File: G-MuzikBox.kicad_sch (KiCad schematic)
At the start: 2 parts, among them IC1 AK4458VN, U1 ORANGE_PI_CM4

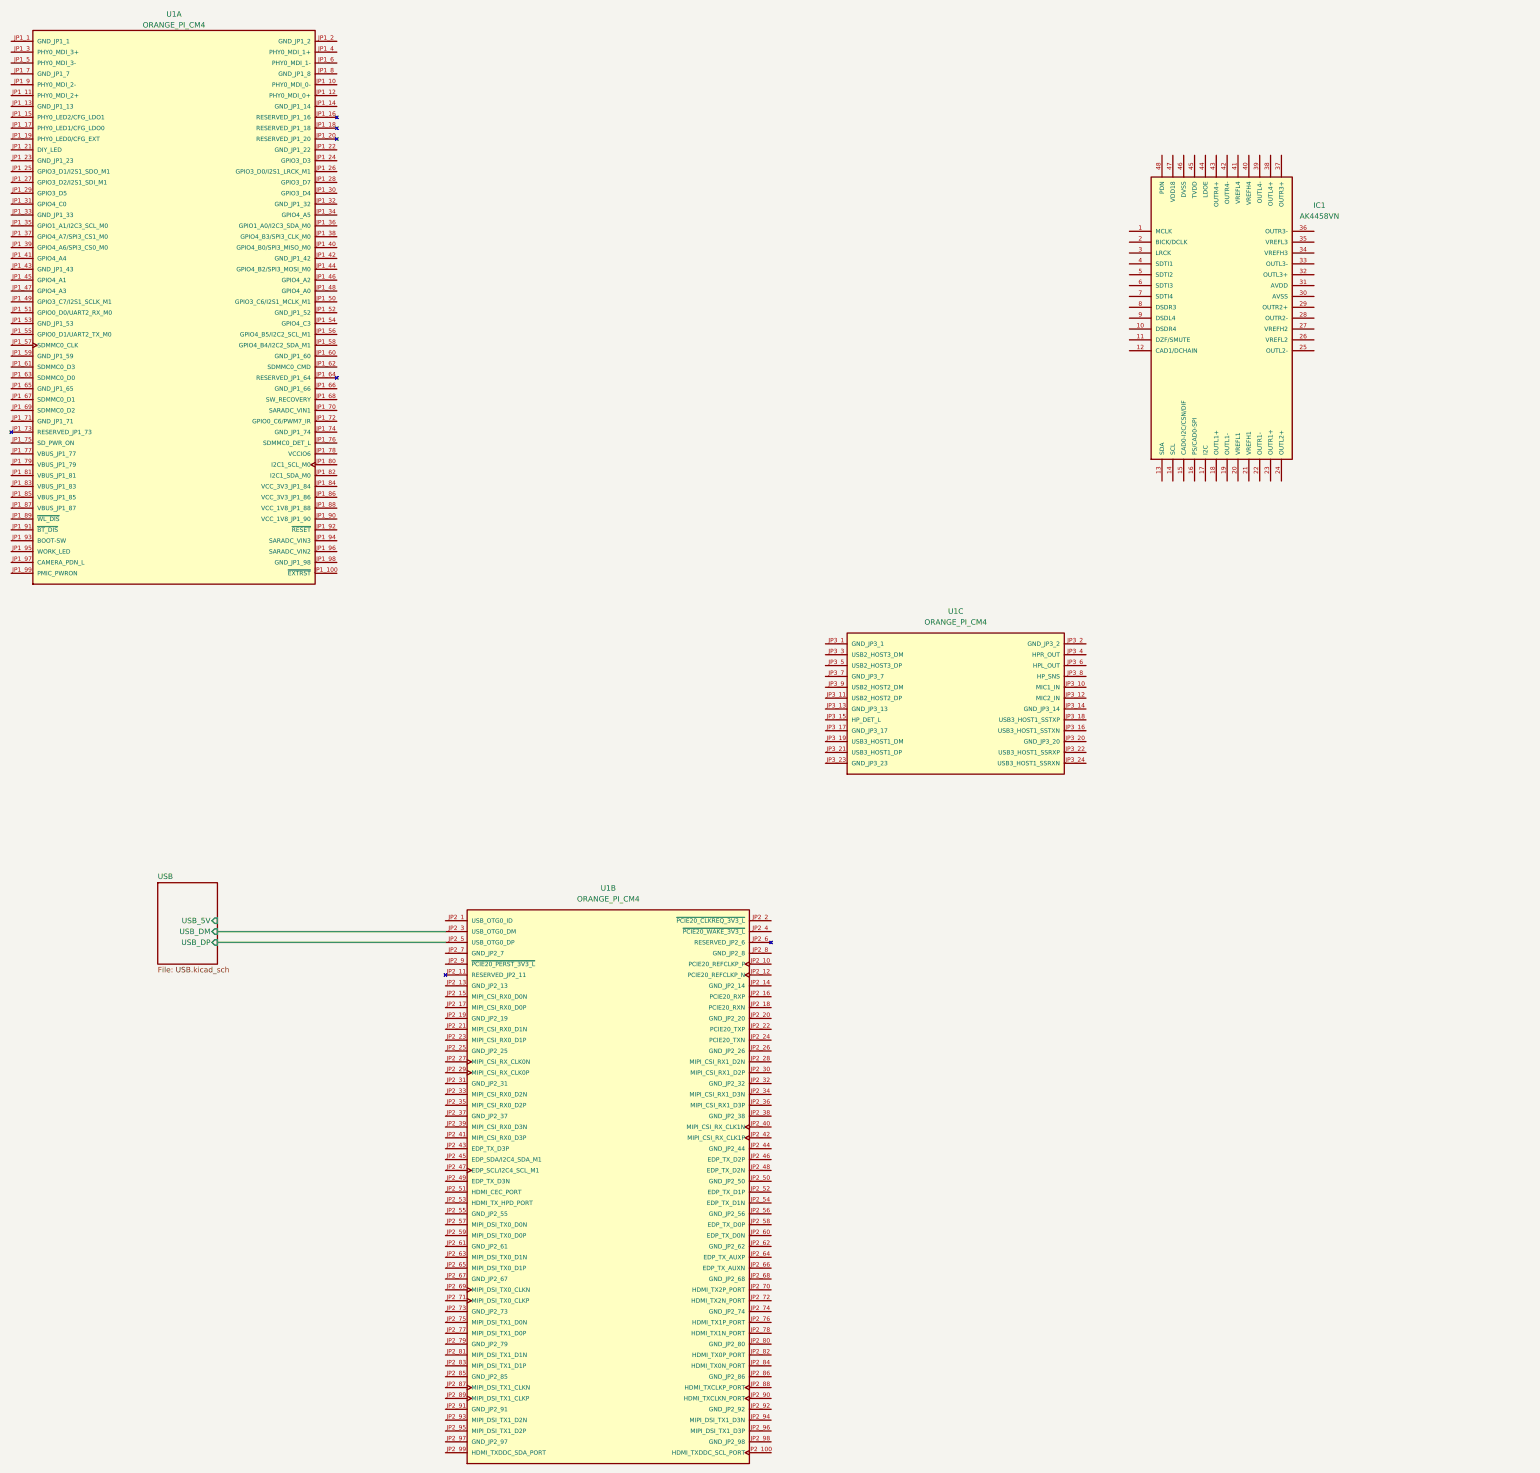
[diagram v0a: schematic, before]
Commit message: dac + lpf + op-amp
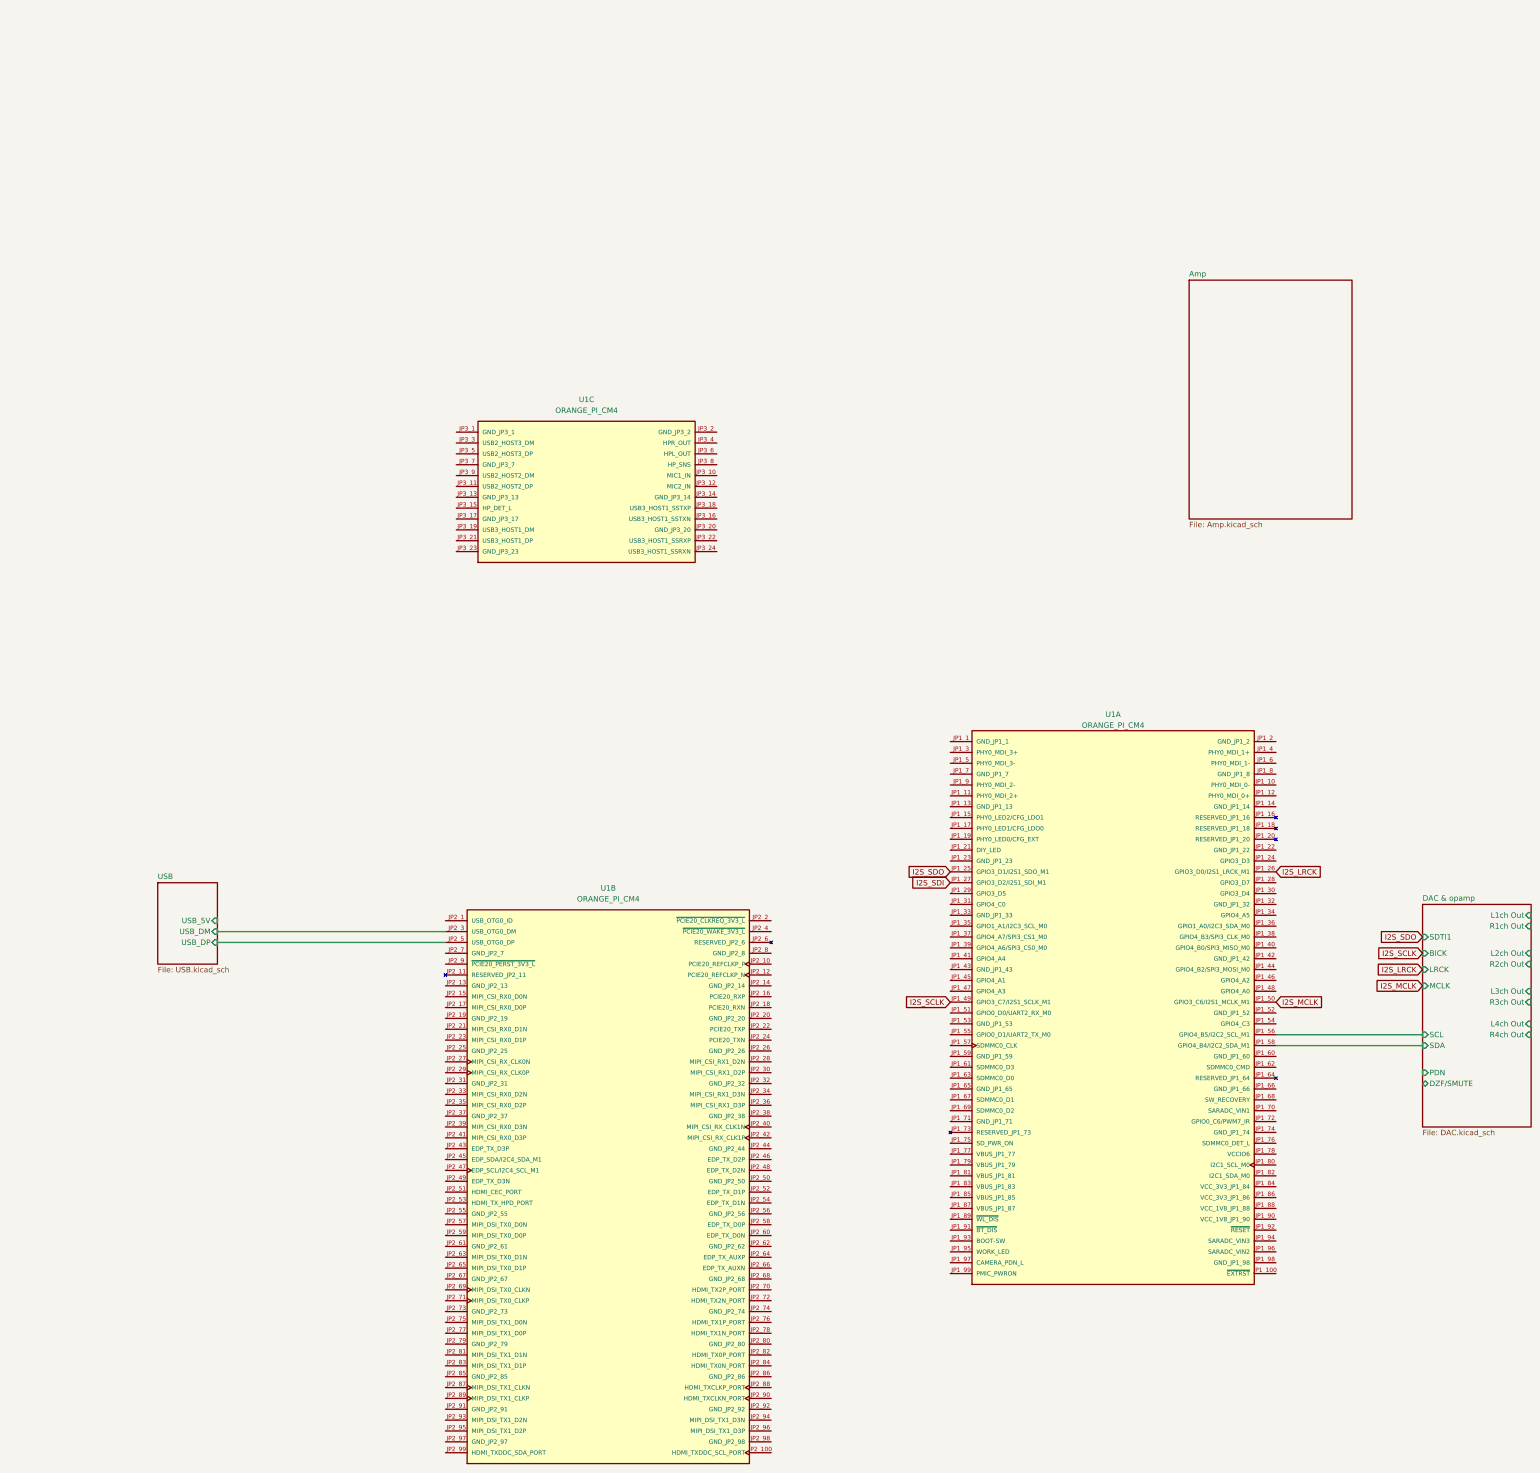
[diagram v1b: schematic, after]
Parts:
- removed IC1: AK4458VN, AK4458VN:QFN50P700X700X100-48N, symbol AK4458VN:AK4458VN
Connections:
- net I2S_SDO: now reaches U1.JP1_25 (GPIO3_D1/I2S1_SDO_M1)
- net I2S_LRCK: now reaches U1.JP1_26 (GPIO3_D0/I2S1_LRCK_M1)
- net I2S_SDI: now reaches U1.JP1_27 (GPIO3_D2/I2S1_SDI_M1)
- net I2S_SCLK: now reaches U1.JP1_49 (GPIO3_C7/I2S1_SCLK_M1)
- net I2S_MCLK: now reaches U1.JP1_50 (GPIO3_C6/I2S1_MCLK_M1)
- net DAC & opamp/SCL: now reaches U1.JP1_56 (GPIO4_B5/I2C2_SCL_M1)
- net DAC & opamp/SDA: now reaches U1.JP1_58 (GPIO4_B4/I2C2_SDA_M1)
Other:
- added sheet Amp (Amp.kicad_sch)
- added sheet DAC & opamp (DAC.kicad_sch)
- moved on the sheet: U1A, U1C
